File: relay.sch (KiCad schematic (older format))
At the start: 3 parts

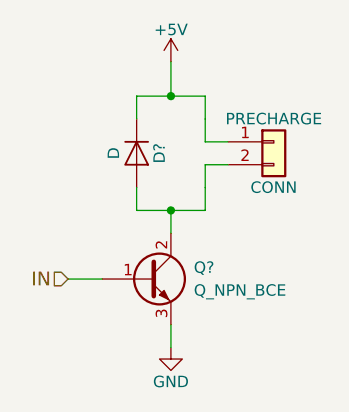
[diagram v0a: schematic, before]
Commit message: Annotate and add negative IOC faults.
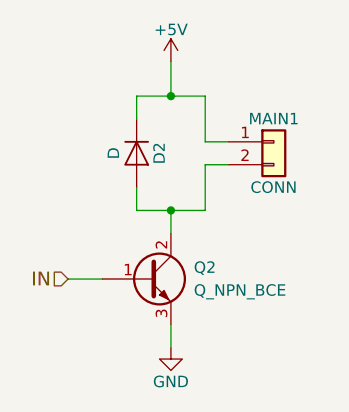
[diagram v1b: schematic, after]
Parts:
- gave numbers to parts that had none: 2
- renumbered PRECHARGE to PRECHARGE1
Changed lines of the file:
@@
 $Descr A4 11693 8268
 encoding utf-8
-Sheet 17 19
+Sheet 18 19
 Title ""
 Date ""
@@
 IN
 $Comp
-L Q_NPN_BCE Q?
+L Q_NPN_BCE Q1
 U 1 1 5B006B25
 P 5750 4000
-AR Path="/5AFF2F49/5AFF30F9/5B006B25" Ref="Q?"  Part="1"
-AR Path="/5AFF2F49/5AFF3733/5B006B25" Ref="Q?"  Part="1"
-F 0 "Q?" H 5950 4050 50  0000 L CNN
+AR Path="/5AFF2F49/5AFF30F9/5B006B25" Ref="Q1"  Part="1"
+AR Path="/5AFF2F49/5AFF3733/5B006B25" Ref="Q2"  Part="1"
+F 0 "Q2" H 5950 4050 50  0000 L CNN
 F 1 "Q_NPN_BCE" H 5950 3950 50  0000 L CNN
 F 2 "" H 5950 4100 50  0001 C CNN
@@
 	5550 4000 5400 4000
 $Comp
-L +5V #PWR?
+L +5V #PWR81
 U 1 1 5B006F20
 P 5850 3050
-AR Path="/5AFF2F49/5AFF30F9/5B006F20" Ref="#PWR?"  Part="1"
-AR Path="/5AFF2F49/5AFF3733/5B006F20" Ref="#PWR?"  Part="1"
-F 0 "#PWR?" H 5850 2900 50  0001 C CNN
+AR Path="/5AFF2F49/5AFF30F9/5B006F20" Ref="#PWR81"  Part="1"
+AR Path="/5AFF2F49/5AFF3733/5B006F20" Ref="#PWR83"  Part="1"
+F 0 "#PWR83" H 5850 2900 50  0001 C CNN
 F 1 "+5V" H 5850 3190 50  0000 C CNN
 F 2 "" H 5850 3050 50  0001 C CNN
@@
 $EndComp
 $Comp
-L GND #PWR?
+L GND #PWR82
 U 1 1 5B006F38
 P 5850 4300
-AR Path="/5AFF2F49/5AFF30F9/5B006F38" Ref="#PWR?"  Part="1"
-AR Path="/5AFF2F49/5AFF3733/5B006F38" Ref="#PWR?"  Part="1"
-F 0 "#PWR?" H 5850 4050 50  0001 C CNN
+AR Path="/5AFF2F49/5AFF30F9/5B006F38" Ref="#PWR82"  Part="1"
+AR Path="/5AFF2F49/5AFF3733/5B006F38" Ref="#PWR84"  Part="1"
+F 0 "#PWR84" H 5850 4050 50  0001 C CNN
 F 1 "GND" H 5850 4150 50  0000 C CNN
 F 2 "" H 5850 4300 50  0001 C CNN
@@
 $EndComp
 $Comp
-L D D?
+L D D1
 U 1 1 5B006F50
 P 5700 3450
-AR Path="/5AFF2F49/5AFF30F9/5B006F50" Ref="D?"  Part="1"
-AR Path="/5AFF2F49/5AFF3733/5B006F50" Ref="D?"  Part="1"
-F 0 "D?" H 5700 3550 50  0000 C CNN
+AR Path="/5AFF2F49/5AFF30F9/5B006F50" Ref="D1"  Part="1"
+AR Path="/5AFF2F49/5AFF3733/5B006F50" Ref="D2"  Part="1"
+F 0 "D2" H 5700 3550 50  0000 C CNN
 F 1 "D" H 5700 3350 50  0000 C CNN
 F 2 "" H 5700 3450 50  0001 C CNN
@@
 	5700 3200 6000 3200
 Wire Wire Line
-	6000 3200 6000 3300
+	6000 3200 6000 3400
 Wire Wire Line
 	5850 3050 5850 3200
@@
 	5700 3600 5700 3700
 Wire Wire Line
-	5700 3700 6000 3700
+	6000 3700 5700 3700
 Wire Wire Line
-	6000 3700 6000 3600
+	6000 3500 6000 3700
 Wire Wire Line
 	5850 3800 5850 3700
@@
 	5850 4200 5850 4300
 $Comp
-L Conn_01x02 PRECHARGE
+L Conn_01x02 PRECHARGE1
 U 1 1 5B007450
 P 6300 3400
-AR Path="/5AFF2F49/5AFF30F9/5B007450" Ref="PRECHARGE"  Part="1"
-AR Path="/5AFF2F49/5AFF3733/5B007450" Ref="MAIN"  Part="1"
-F 0 "PRECHARGE" H 6300 3500 50  0000 C CNN
+AR Path="/5AFF2F49/5AFF30F9/5B007450" Ref="PRECHARGE1"  Part="1"
+AR Path="/5AFF2F49/5AFF3733/5B007450" Ref="MAIN1"  Part="1"
+F 0 "MAIN1" H 6300 3500 50  0000 C CNN
 F 1 "CONN" H 6300 3200 50  0000 C CNN
 F 2 "" H 6300 3400 50  0001 C CNN
@@
 $EndComp
 Wire Wire Line
-	6000 3300 6000 3400
-Wire Wire Line
 	6000 3400 6100 3400
 Wire Wire Line
 	6100 3500 6000 3500
-Wire Wire Line
-	6000 3600 6000 3500
 $EndSCHEMATC
